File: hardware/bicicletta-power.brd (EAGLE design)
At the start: 160 x 100 mm, 20 parts, among them IC1 LM5017

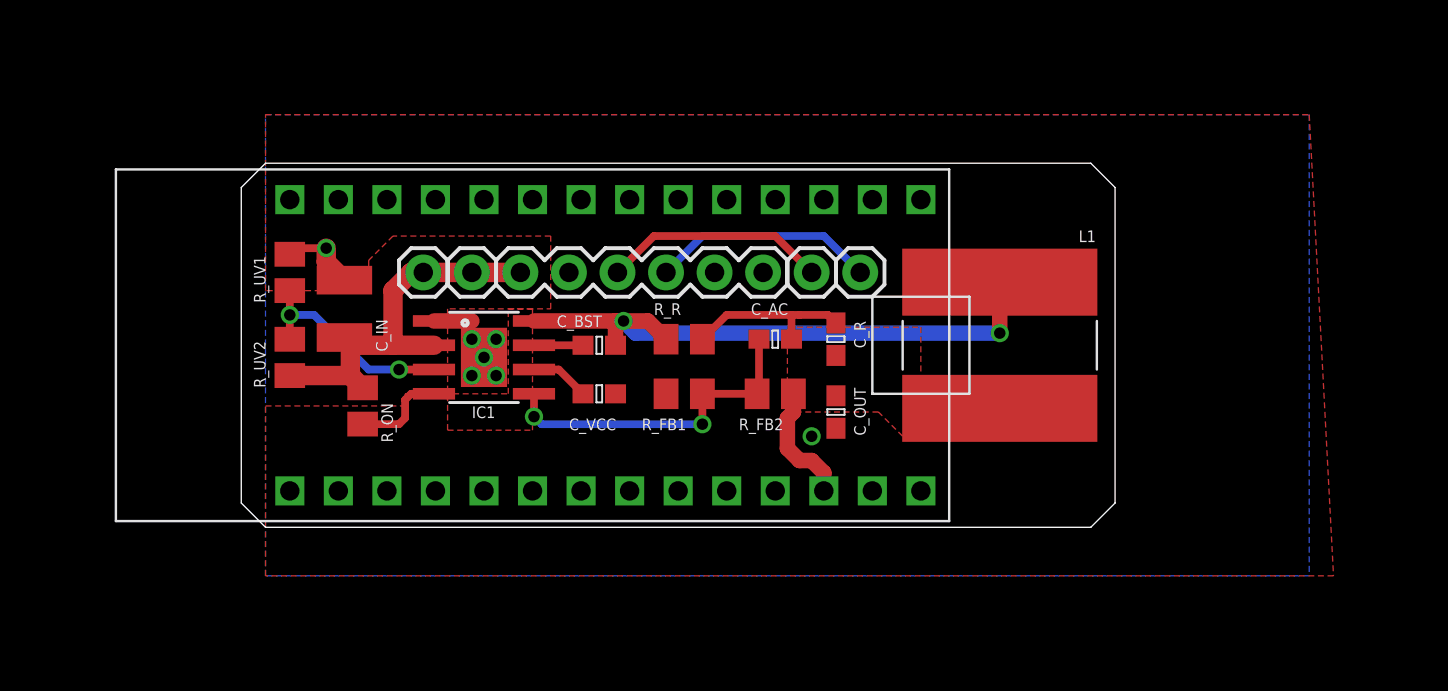
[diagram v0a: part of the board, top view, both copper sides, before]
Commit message: There it is. Order that.
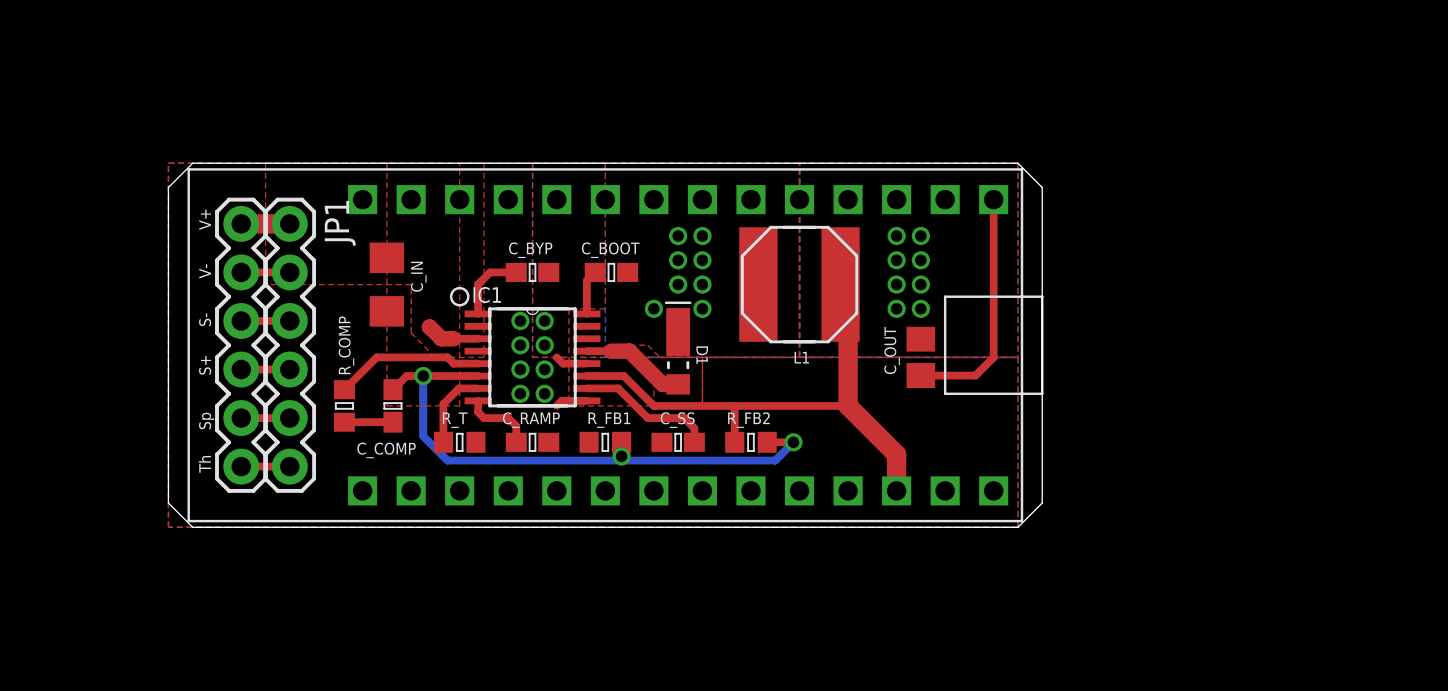
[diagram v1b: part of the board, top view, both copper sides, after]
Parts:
- removed C_AC: 100nF, rcl:C0603
- removed C_BST: 0.01uF, rcl:C0603
- removed C_R: 3300pF, rcl:C0603
- removed C_VCC: 1uF, rcl:C0603
- removed JP4, JP5, JP6, JP7: M01PTH, SparkFun-Connectors:1X01
- removed R_ON: 250K, rcl:M0805
- removed R_R: 2M, rcl:M0805
- removed R_UV1: 14K, rcl:M0805
- removed R_UV2: 125K, rcl:M0805
- added C_BOOT: 22nF, rcl:C0603
- added C_BYP: 1uF, rcl:C0603
- added C_COMP: 1.8nF, rcl:C0603
- added C_RAMP: 470pF, rcl:C0603
- added C_SS: 1nF, rcl:C0603
- added D1: DFLS1100-7, TI:POWERDI123
- added JP1: (no value), SparkFun-Connectors:1X06
- added R_COMP: 19K1, rcl:R0603
- added R_T: 10K7 75V, rcl:R0603
- C_IN: value 2.2uF -> 1uF; device rcl:C1210K -> rcl:C1206
- C_OUT: value 5.6uF -> 10uF; device rcl:C0603 -> rcl:C0805
- IC1: value LM5017 -> LM5574MT/NOPB; device Railstars:SOIC-8-POWERPAD -> TI:MTC16
- L1: value 100uH -> SRN6045-101M; device Railstars:SRN1060 -> TI:SRN6045
- R_FB1: device rcl:M0805 -> rcl:R0603
- R_FB2: value 3K -> 3K09; device rcl:M0805 -> rcl:R0603
- moved JP3 14.8 mm to (40.6, 80.6), turned to 270 degrees
- moved L1 10.9 mm to (69.8, 77.5)
- moved C_OUT 5.28 mm to (76.2, 73.7)
- moved R_FB1 4.85 mm to (59.7, 69.2)
- moved U$1 3.81 mm to (59.7, 74.3)
- moved R_FB2 2.84 mm to (67.3, 69.2), turned to 180 degrees
- moved C_IN 2.56 mm to (48.3, 77.5), turned to 270 degrees
- moved IC1 2.54 mm to (55.9, 73.7), turned to 0 degrees
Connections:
- removed net N$4: C_BST.2, IC1.8, L1.P$1, R_R.1
- new net N$10: C_BOOT.1, IC1.16
- new net N$11: C_BOOT.2, D1.K, IC1.14, IC1.15, L1.1
- new net N$5: IC1.7, R_T.1
- new net N$8: IC1.5, R_COMP.1
- net 5V: now also IC1.11, L1.2; no longer C_R.2, L1.P$2
- net GND: now also C_BYP.2, C_RAMP.2, C_SS.2, IC1.12, IC1.9, JP1.2, R_T.2; no longer C_VCC.2, IC1.1, IC1.P$1, R_UV1.1
- net N$1: now also C_SS.1, IC1.10; no longer IC1.4, R_ON.2
- net N$2: now also C_BYP.1, IC1.1; no longer C_AC.2, IC1.5, R_FB1.2, R_FB2.1
- net N$3: now also C_RAMP.1, IC1.8; no longer IC1.3, R_UV1.2, R_UV2.2
- net N$6: now also C_COMP.2, IC1.6, R_FB1.2, R_FB2.1; no longer C_AC.1, C_R.1, R_R.2
- net N$7: now also C_COMP.1, R_COMP.2; no longer C_BST.1, IC1.7
- net N$9: now also D1.A, IC1.13; no longer C_VCC.1, IC1.6
- net SHUNT+: now also JP1.4; no longer JP4.1
- net SHUNT-: now also JP1.3; no longer JP5.1
- net SPEED_5: now also JP1.5
- net THROTTLE_OUT_5: now also JP1.6
- net V_BATT: now also IC1.3, JP1.1; no longer IC1.2, JP6.1, JP7.1, R_ON.1, R_UV2.1
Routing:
- net N$4: track 31.2 -> 0.00 mm, vias 2 -> 0
- net N$6: track 8.96 -> 30.4 mm, vias 0 -> 3
- net 5V: track 6.37 -> 25.5 mm, vias 0 -> 8
- net V_BATT: track 21.0 -> 5.35 mm
- net N$2: track 17.5 -> 3.80 mm, vias 2 -> 0
- net GND: track 7.23 -> 18.4 mm, vias 7 -> 8
- net SHUNT+: track 11.7 -> 2.54 mm
- net SHUNT-: track 11.7 -> 2.54 mm
- net N$8: track 0.00 -> 7.83 mm
- net N$3: track 11.3 -> 3.74 mm, vias 2 -> 0
- net N$5: track 0.00 -> 4.16 mm
- net THROTTLE_OUT_5: track 0.00 -> 2.54 mm
- net SPEED_5: track 0.00 -> 2.54 mm
- net N$9: track 3.09 -> 5.49 mm
- net N$10: track 0.00 -> 2.35 mm
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- added copper zone on layer 16, net 5V
- added copper zone on layer 1, net N$11
- added copper zone on layer 16, net N$11
- added copper zone on layer 1, net N$9
- added copper zone on layer 1, net V_BATT
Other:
- outline, holes or cut-outs redrawn
- board text added: "S+"
- board text added: "S-"
- board text added: "Sp"
- board text added: "Th"
- board text added: "V+"
- board text added: "V-"
